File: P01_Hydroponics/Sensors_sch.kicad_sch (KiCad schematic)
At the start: 9 parts, among them J2 JST_PH_3P_TEMP, J3 JST_PH_3P_FLOW, J4 JST_PH_3P_WLS1, J5 JST_PH_4P_WLS0, J6 JST_PH_2P_PUMP, Q2 NMOS

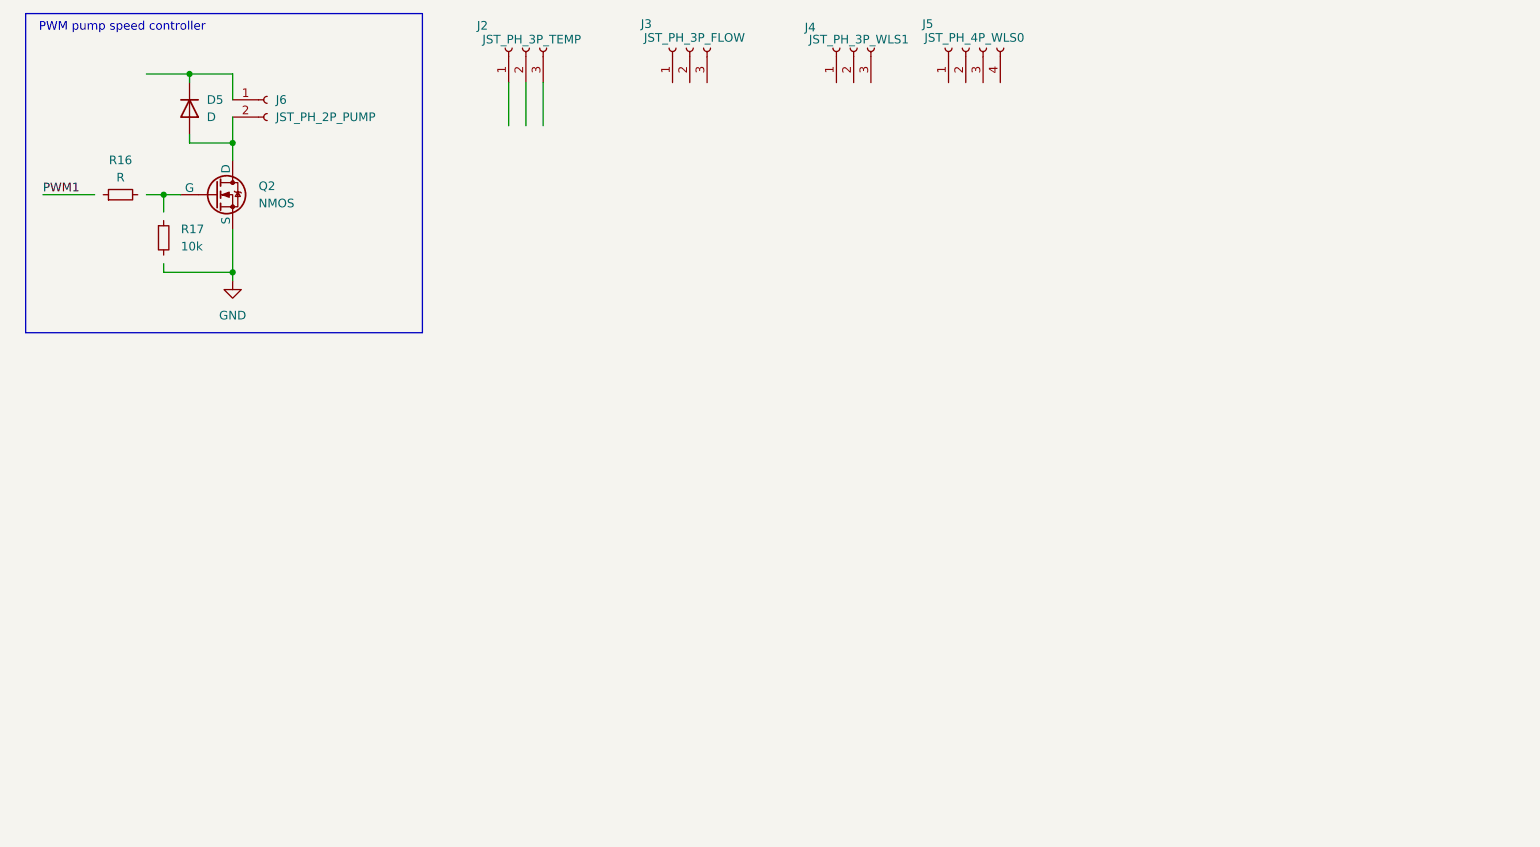
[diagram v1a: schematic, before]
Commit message: Need review
Please review the schematics.
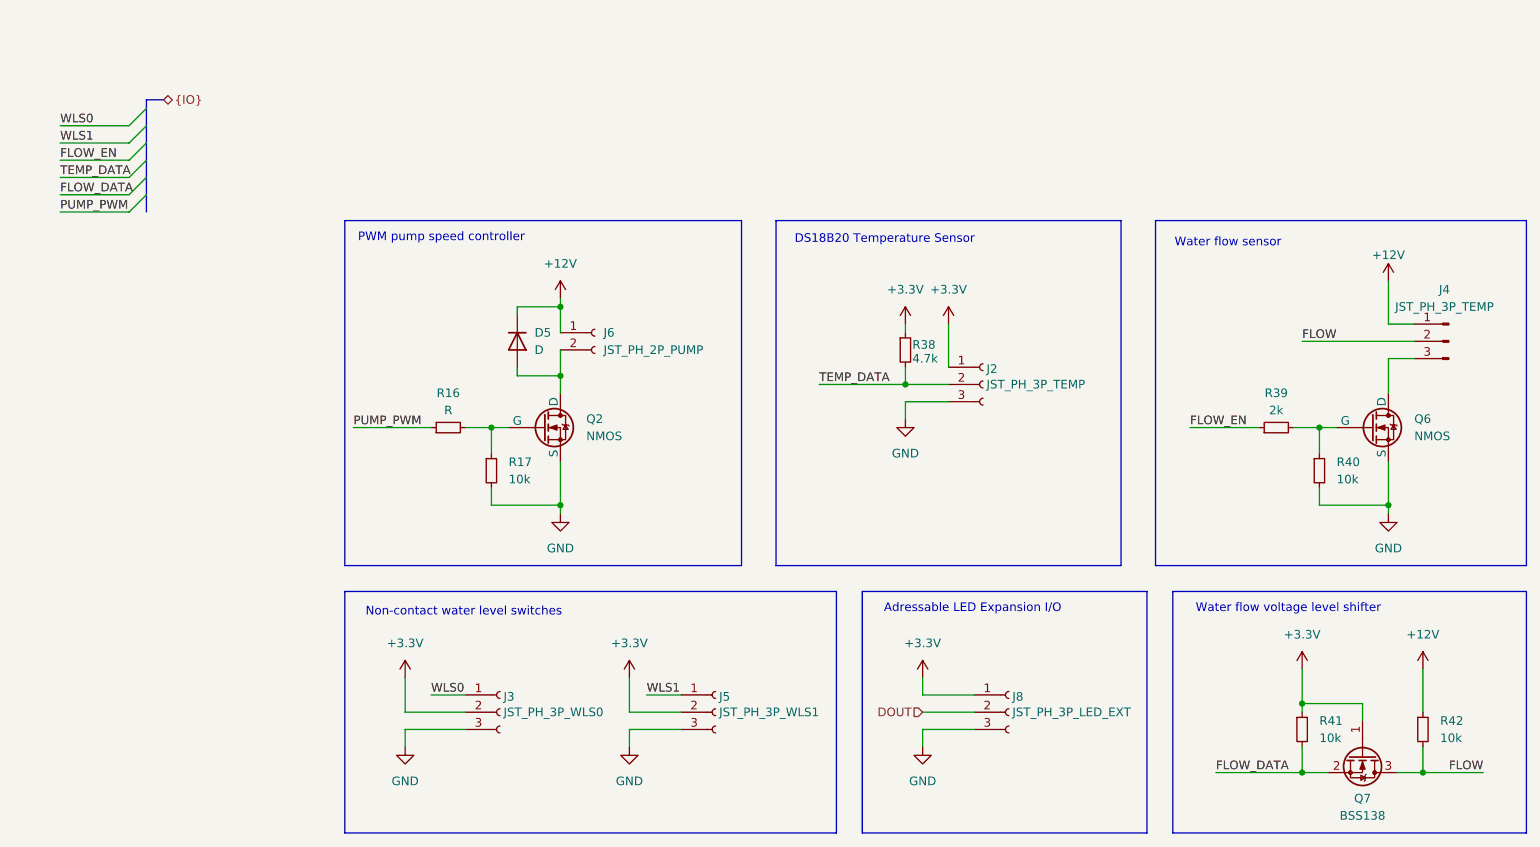
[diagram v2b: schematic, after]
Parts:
- removed J4: JST_PH_3P_WLS1, symbol Connector:Conn_01x03_Socket
- removed J5: JST_PH_4P_WLS0, symbol Connector:Conn_01x04_Socket
- added J4: JST_PH_3P_TEMP, symbol Connector:Conn_01x03_Pin
- added J5: JST_PH_3P_WLS1, symbol Connector:Conn_01x03_Socket
- added J8: JST_PH_3P_LED_EXT, symbol Connector:Conn_01x03_Socket
- added Q6: NMOS, symbol Simulation_SPICE:NMOS
- added Q7: BSS138, Package_TO_SOT_SMD:SOT-23, symbol Transistor_FET:BSS138
- added R38: 4.7k, symbol Device:R_Small
- added R39: 2k, symbol Device:R_Small
- added R40, R41, R42: 10k, symbol Device:R_Small
- J3: value JST_PH_3P_FLOW -> JST_PH_3P_WLS0
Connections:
- net GND: now also J2.3 (Pin_3), J3.3 (Pin_3), R17.2, J5.3 (Pin_3), J8.3 (Pin_3), Q6.3 (S), R40.2
- net at R17.1: now also Q2.2 (G), R16.2
- net +3.3V: now reaches J2.1 (Pin_1)
- net +3.3V: now also J3.2 (Pin_2), J5.2 (Pin_2), J8.1 (Pin_1), Q7.1 (G), R38.1, R41.1
- net TEMP_DATA: now reaches J2.2 (Pin_2)
- net TEMP_DATA: now also R38.2
- net +12V: now reaches D5.1 (K), J6.1 (Pin_1)
- net +12V: now also J4.1 (Pin_1), R42.1
- net WLS0: now reaches J3.1 (Pin_1)
- net PUMP_PWM: now reaches R16.1
- new net: Q6.2 (G), R39.2, R40.1
- new net: J4.3 (Pin_3), Q6.1 (D)
- new net DOUT: J8.2 (Pin_2)
- new net FLOW: J4.2 (Pin_2), Q7.3 (D), R42.2
- new net FLOW_DATA: Q7.2 (S), R41.2
- new net FLOW_EN: R39.1
- new net WLS1: J5.1 (Pin_1)
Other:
- note added: "Adressable LED Expansion I/O"
- note added: "DS18B20 Temperature Sensor"
- note added: "Non-contact water level switches"
- note added: "Water flow sensor"
- note added: "Water flow voltage level shifter"
- moved on the sheet: D5, J2, J6, Q2, R16, R17
